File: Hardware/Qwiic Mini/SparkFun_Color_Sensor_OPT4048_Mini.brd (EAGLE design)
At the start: 25.4 x 12.7 mm, 51 parts, among them J4 QWIIC_RIGHT_ANGLE, J5 QWIIC_RIGHT_ANGLE, U1 OPT4048

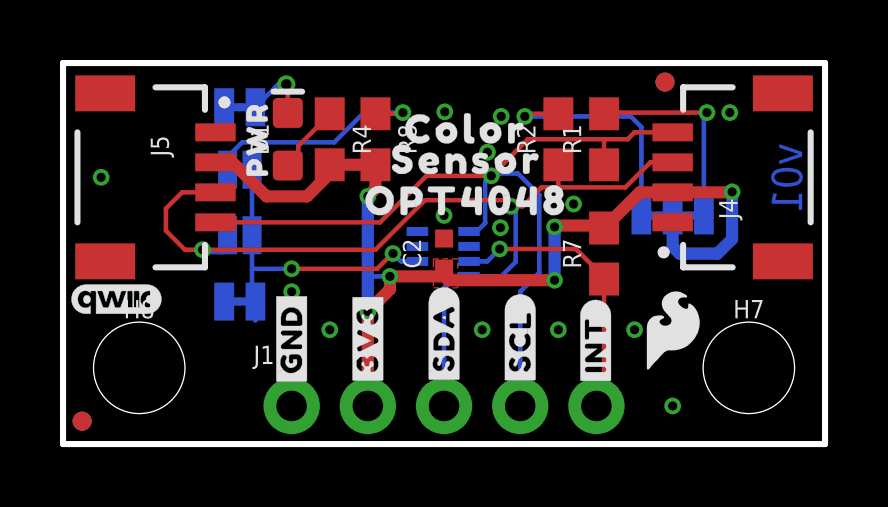
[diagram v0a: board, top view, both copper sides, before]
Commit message: Approves some DRC errors
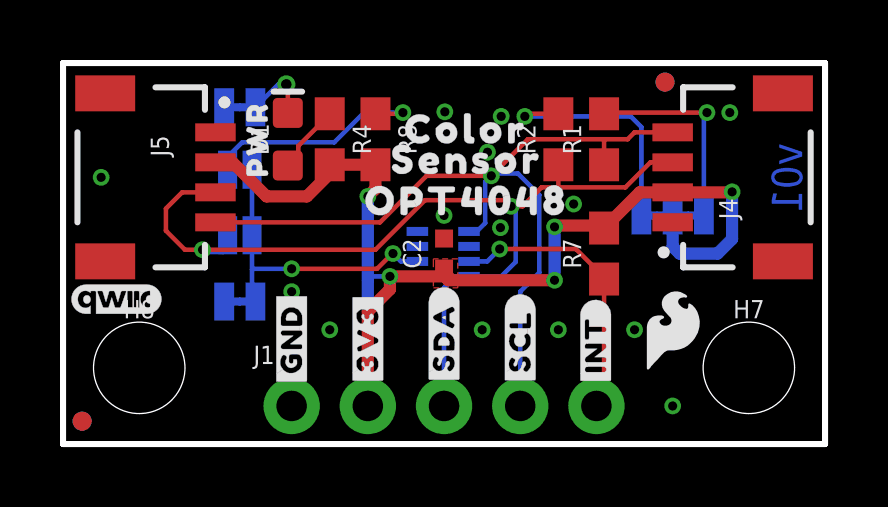
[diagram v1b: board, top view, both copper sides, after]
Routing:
- net ADDR: track 10.9 -> 10.3 mm
- net 3.3V: vias 6 -> 5
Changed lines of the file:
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@@
 <wire x1="21.8186" y1="6.35" x2="22.3012" y2="6.8326" width="0.4064" layer="16"/>
 <wire x1="8.89" y1="9.31" x2="10.414" y2="9.31" width="0.4064" layer="1"/>
-<via x="10.16" y="4.4196" extent="1-16" drill="0.3048"/>
 <wire x1="10.16" y1="5.461" x2="10.16" y2="4.4196" width="0.4064" layer="16"/>
 <wire x1="8.89" y1="9.017" x2="8.89" y2="9.31" width="0.4064" layer="1"/>
@@
 <contactref element="0X45" pad="1"/>
 <contactref element="0X46" pad="1"/>
-<wire x1="6.4135" y1="4.1148" x2="6.4135" y2="4.7498" width="0.1524" layer="16"/>
 <wire x1="6.4135" y1="4.7498" x2="6.2992" y2="4.8641" width="0.1524" layer="16"/>
 <wire x1="6.2992" y1="4.8641" x2="6.2992" y2="5.8166" width="0.1524" layer="16"/>
